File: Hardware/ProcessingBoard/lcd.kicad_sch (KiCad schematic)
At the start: 22 parts, among them J700 TXW280064B0-R, J701 Conn_01x09, U700 CAT4139

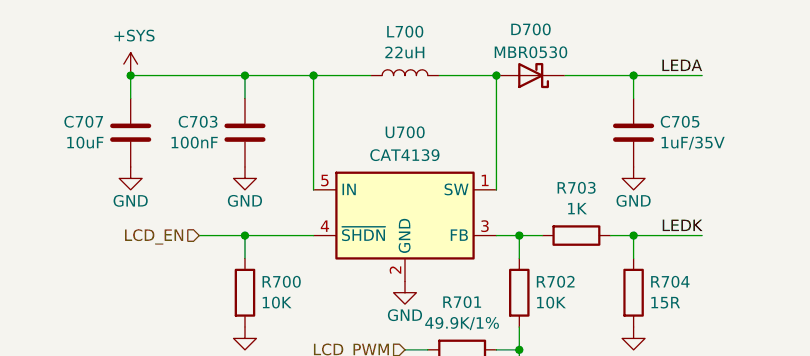
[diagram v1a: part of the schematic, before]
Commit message: pcb: PB r0p2 and CB r0p3 freeze
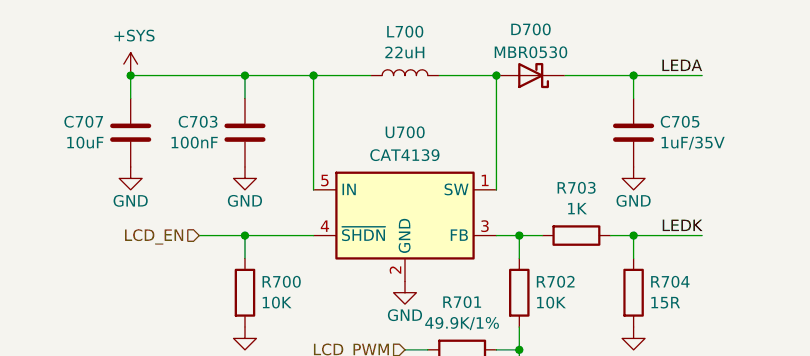
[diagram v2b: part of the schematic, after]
